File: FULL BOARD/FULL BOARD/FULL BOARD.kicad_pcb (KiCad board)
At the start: 2 copper layers, 101 parts, among them IC1 TAS5760LDAP, J1 PJ-036AH-SMT-TR, J2 Micro_SD_Card, J3 B2B-PH-K-S, J4 5019514000, J5 61201021621, J6 B2B-PH-K-S, SW1 SW_Push, U1 LD1117S33TR_SOT223, U2 STM32H743VITx, Y1 ABLS7M2-16.000MHZ-D-2Y-T

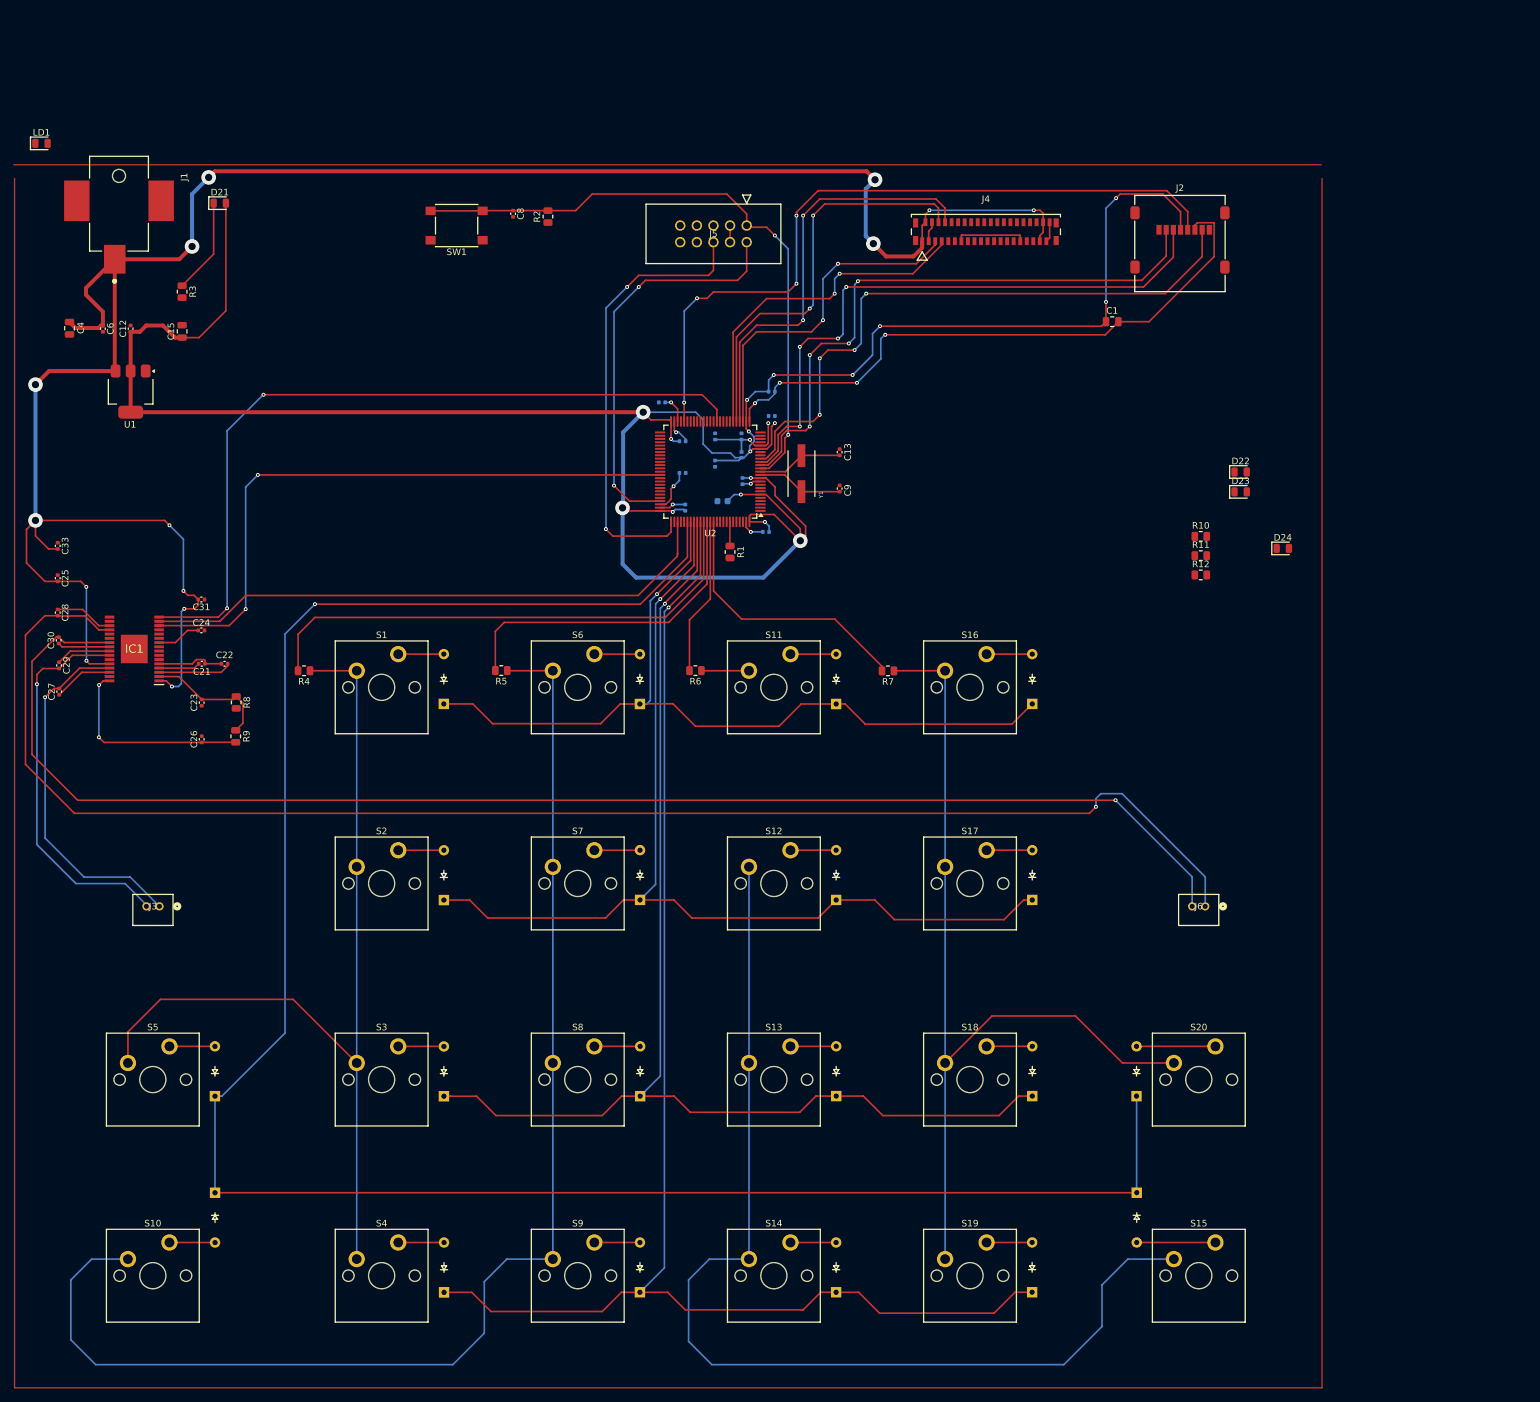
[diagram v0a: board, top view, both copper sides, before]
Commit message: final(?) PCB before presentation
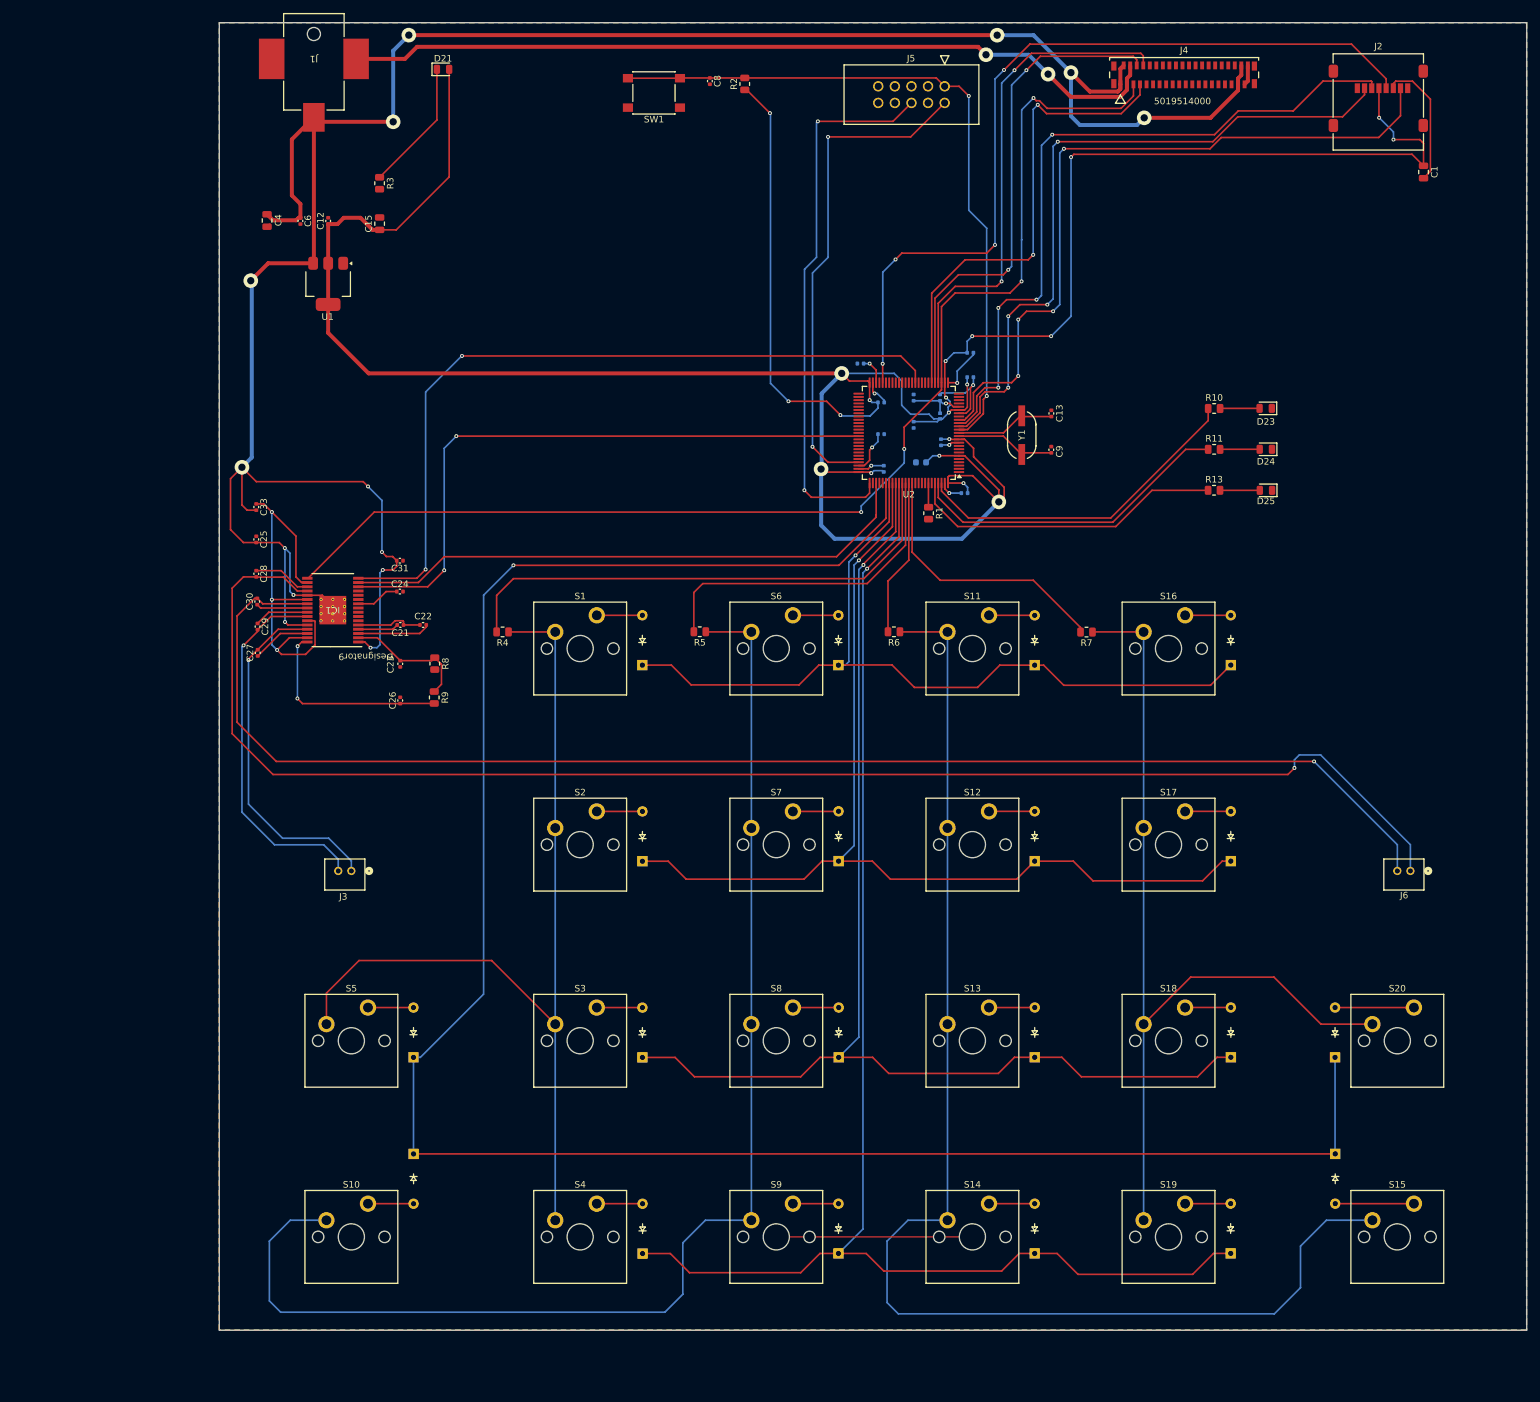
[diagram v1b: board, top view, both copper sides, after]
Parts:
- removed D22: LED, LED_SMD:LED_0805_2012Metric
- removed LD1: LED_Green, LED_SMD:LED_0805_2012Metric
- removed R12: 10k, Resistor_SMD:R_0805_2012Metric
- added D25: LED, LED_SMD:LED_0805_2012Metric, F.Cu at (211.0, 30.3)
- added R13: 10k, Resistor_SMD:R_0805_2012Metric, F.Cu at (203.1, 30.3)
- D1, D10, D11, D12, D13, D14, D15, D16, D17, D18, D19, D2, D20, D3, D4, D5, D6, D7, D8, D9: footprint Keyboard footprint:Diode_DO-35 -> ScottoKeebs_Components:Diode_DO-35
- FL1: footprint footprints:BEADC1005X55N -> Ferrite Bead:BEADC1005X55N
- IC1: footprint KiCad:SOP65P810X120-33N -> Audio Amp:DAP0032A_M
- J1: footprint PJ-036AH-SMT-TR:CUI_PJ-036AH-SMT-TR -> power jack:CONN3_PJ-036AH_CUD
- J3, J6: footprint audiojack:CONN2_B2B-PH-K-S_JST -> Audio Jack:CONN2_B2B-PH-K-S_JST
- J4: footprint footprints:CON_5019514000 -> Ribbon Connector:CON_5019514000
- J5: footprint footprints:CONN_61201021621_WRE -> Debugger:CONN_61201021621_WRE
- S1, S10, S11, S12, S13, S14, S15, S16, S17, S18, S19, S2, S20, S3, S4, S5, S6, S7, S8, S9: footprint Keyboard footprint:MX_PCB_1.00u -> ScottoKeebs_MX:MX_PCB_1.00u
- Y1: footprint footprints:XTAL_ABLS7M2-16.000MHZ-D-2Y-T -> crystal osc:XTAL_ABLS7M2_ABR
- moved C1 52.8 mm to (235.1, -18.4), turned to -90 degrees
- moved J1 42.9 mm to (65.4, -35.2), turned to 180 degrees
- moved D21 39.8 mm to (85.1, -34.1)
- moved J4 38.7 mm to (198.5, -33.2)
- moved J2 37.3 mm to (228.2, -29.1)
- moved J5 37.0 mm to (161.9, -31.5)
- moved SW1 36.4 mm to (117.4, -30.4)
- moved C8 36.3 mm to (125.9, -32.3)
- moved R2 36.3 mm to (131.3, -31.8)
- moved R3 34.5 mm to (75.4, -16.6)
- moved C15 34.4 mm to (75.4, -10.4)
- moved C4 34.4 mm to (58.2, -10.9)
- moved C12 34.4 mm to (67.6, -10.9)
- moved C6 34.4 mm to (63.3, -10.9)
- moved U1 34.4 mm to (67.6, -1.24)
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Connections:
- IC1 pad 33: unconnected-(IC1-EP-Pad33) -> +5V
- U2 pad 1: Net-(U2-PE2) -> unconnected-(U2-PE2-Pad1)
- U2 pad 96: unconnected-(U2-PB9-Pad96) -> Net-(U2-PB9)
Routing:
- net I2S_WS: track 51.7 -> 186.5 mm, vias 2 -> 4
- net GND: track 128.7 -> 245.0 mm, vias 8 -> 11
- net +3.3V: track 382.7 -> 485.4 mm, vias 17 -> 20
- net Net-(U2-PE1): track 0.00 -> 51.7 mm
- net Net-(U2-PE0): track 0.00 -> 49.7 mm
- net Net-(U2-PB9): track 0.00 -> 48.7 mm
- net +5V: track 337.5 -> 378.2 mm
- net Net-(R6-Pad1): track 173.4 -> 201.9 mm
- net /LCD_MOSI: track 53.0 -> 73.9 mm
- net /SD_DO: track 95.2 -> 111.3 mm
- net /SWC: track 69.2 -> 85.0 mm
- net /SD_DI: track 92.8 -> 107.9 mm
- net /SD_CLK: track 112.0 -> 126.8 mm
- net /SWDIO: track 61.9 -> 76.4 mm
- net /LCD_SCK: track 64.7 -> 78.7 mm
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- added copper zone on B.Cu, net GND
- added copper zone on F.Cu, net GND
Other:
- board outline added: 200 x 200 mm
